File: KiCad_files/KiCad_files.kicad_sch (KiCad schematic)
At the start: 87 parts, among them J1 Conn_01x02_Socket, J10 MB1, J10 MB2, J13 MB1, J14 MB1, J16 MB2, J3 Conn_01x03_Socket, J6 Conn_01x01_Socket, J7 Conn_01x01_Socket, J8 Conn_01x01_Socket, J8 MB1, J8 MB2, J9 Conn_01x01_Socket, J9 MB1, J9 MB2, SW1 SW_Omron_B3FS, U2 LM22670QMR-5.0, U3 MC33275ST-3.3T3G, U4 ADM3488ExR, U6 LT1789

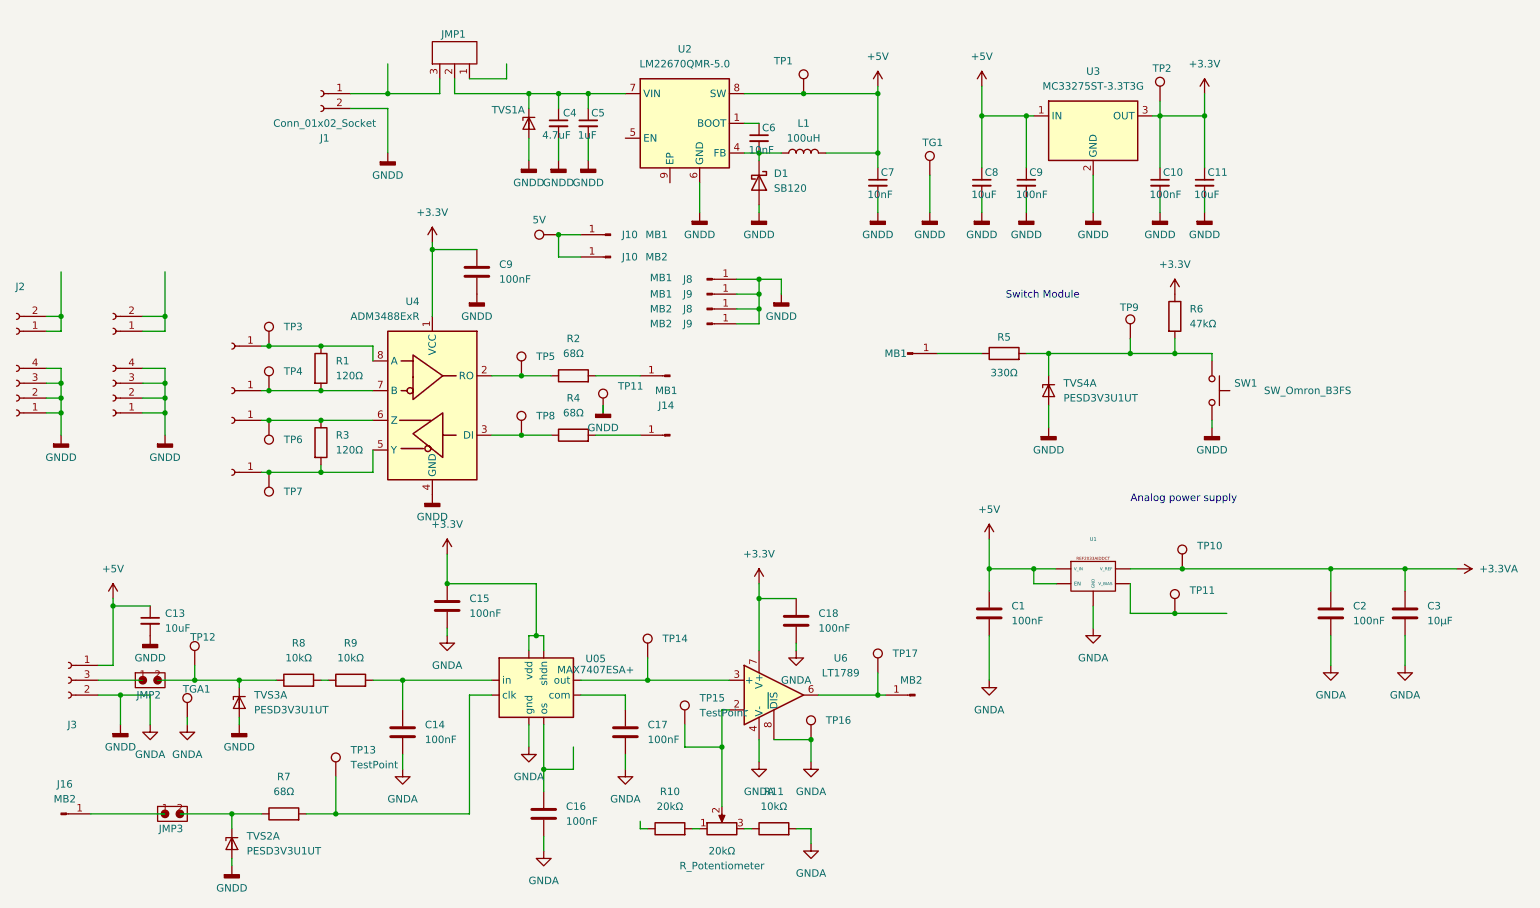
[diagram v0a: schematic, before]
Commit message: i inserted some footprints
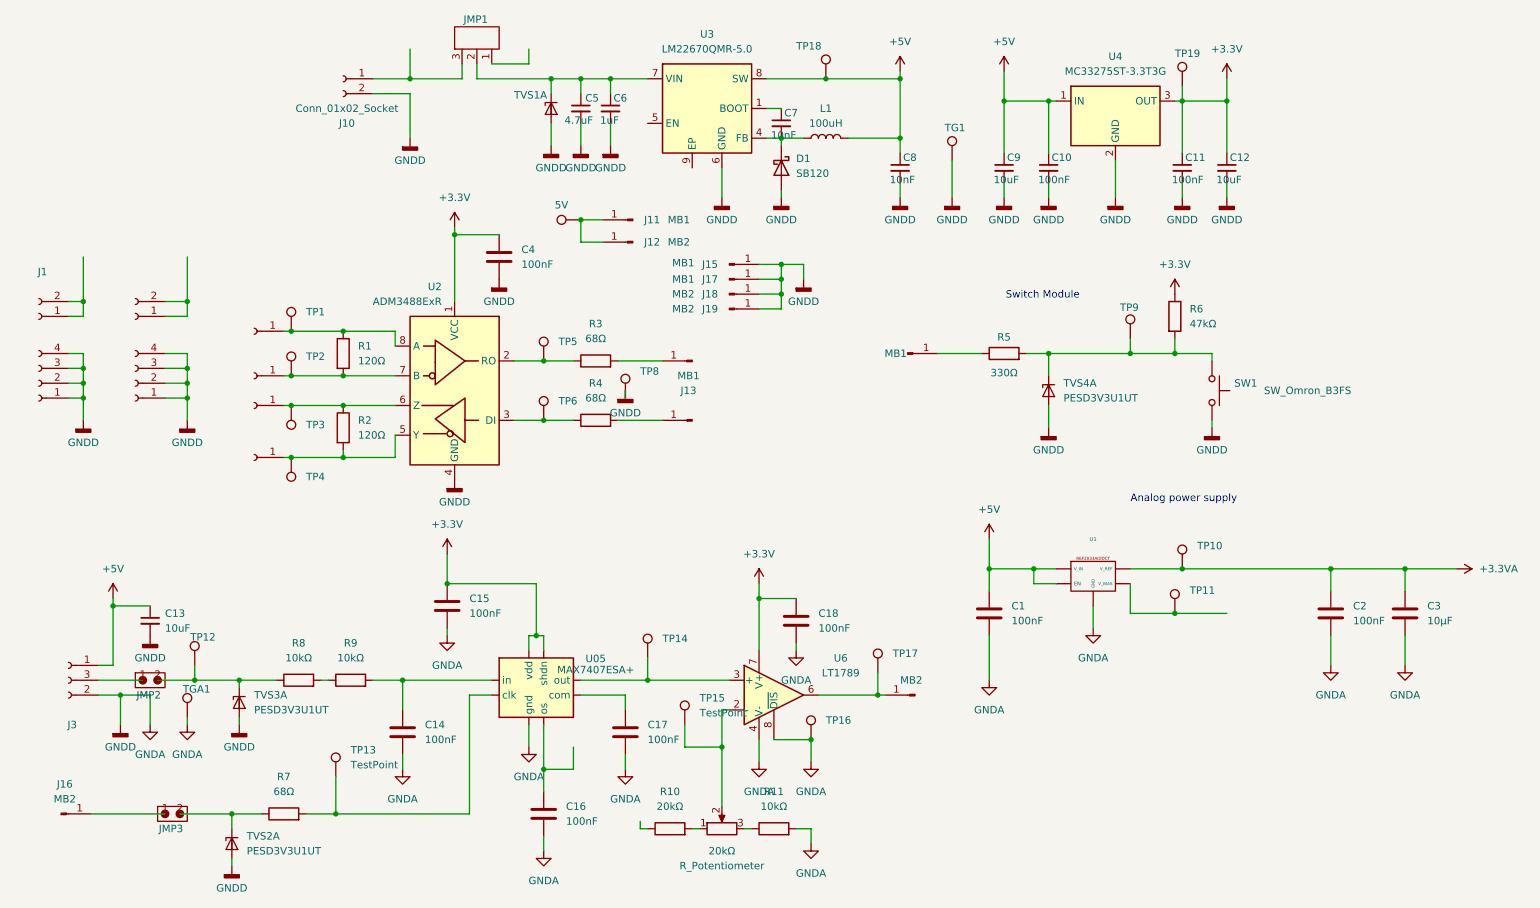
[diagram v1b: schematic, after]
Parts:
- removed C4: 4.7uF, symbol Device:C_Small
- removed C9: 100nF, symbol Device:C
- removed J10, J8, J9: MB1, symbol Connector:Conn_01x01_Pin
- removed J10, J8, J9: MB2, symbol Connector:Conn_01x01_Pin
- removed J2: ~, symbol Connector:Conn_01x02_Socket
- removed J3: ~, symbol Connector:Conn_01x04_Socket
- removed TP11: TestPoint, symbol Connector:TestPoint
- removed U2: LM22670QMR-5.0, Package_SO:SOIC-8-1EP_3.9x4.9mm_P1.27mm_EP2.29x3mm, symbol Regulator_Switching:LM22676MR-5
- removed U3: MC33275ST-3.3T3G, Package_TO_SOT_SMD:SOT-223, symbol Regulator_Linear:LT1963AxST-3.3
- removed U4: ADM3488ExR, Package_SO:SOIC-8_3.9x4.9mm_P1.27mm, symbol Interface_UART:ADM3488ExR
- added C12: 10uF, Capacitor_SMD:C_1210_3225Metric_Pad1.33x2.70mm_HandSolder, symbol Device:C_Small
- added C4: 100nF, symbol Device:C
- added J10: Conn_01x02_Socket, symbol Connector:Conn_01x02_Socket
- added J11, J15, J17: MB1, symbol Connector:Conn_01x01_Pin
- added J12, J18, J19: MB2, symbol Connector:Conn_01x01_Pin
- added J2: ~, symbol Connector:Conn_01x04_Socket
- added TP19: TestPoint, symbol Connector:TestPoint
- added U2: ADM3488ExR, Package_SO:SOIC-8_3.9x4.9mm_P1.27mm, symbol Interface_UART:ADM3488ExR
- added U3: LM22670QMR-5.0, Package_SO:SOIC-8-1EP_3.9x4.9mm_P1.27mm_EP2.29x3mm, symbol Regulator_Switching:LM22676MR-5
- added U4: MC33275ST-3.3T3G, Package_TO_SOT_SMD:SOT-223, symbol Regulator_Linear:LT1963AxST-3.3
- C10, C7: footprint (none) -> Capacitor_SMD:C_1206_3216Metric_Pad1.33x1.80mm_HandSolder
- C11: value 10uF -> 100nF; footprint (none) -> Capacitor_SMD:C_1206_3216Metric_Pad1.33x1.80mm_HandSolder
- C5: value 1uF -> 4.7uF; footprint (none) -> Capacitor_SMD:C_1206_3216Metric_Pad1.33x1.80mm_HandSolder
- C6: value 10nF -> 1uF; footprint (none) -> Capacitor_SMD:C_1206_3216Metric_Pad1.33x1.80mm_HandSolder
- C8: value 10uF -> 10nF; footprint (none) -> Capacitor_SMD:C_1206_3216Metric_Pad1.33x1.80mm_HandSolder
- C9: value 100nF -> 10uF; footprint (none) -> Capacitor_SMD:C_1210_3225Metric_Pad1.33x2.70mm_HandSolder
- J1: value Conn_01x02_Socket -> ~
- JMP1: footprint (none) -> Jumper:Pin_Header_2x1_P2.54mm_Vertical
- R1, R4: footprint (none) -> Resistor_SMD:R_1206_3216Metric_Pad1.30x1.75mm_HandSolder
- R2: value 68Ω -> 120Ω; footprint (none) -> Resistor_SMD:R_1206_3216Metric_Pad1.30x1.75mm_HandSolder
- R3: value 120Ω -> 68Ω; footprint (none) -> Resistor_SMD:R_1206_3216Metric_Pad1.30x1.75mm_HandSolder
- TP18: value 5V -> TestPoint
- TP7: value TestPoint -> 5V
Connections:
- net +3.3V: now also C12.1, C4.1, TP19.1, U2.1 (VCC), U4.3 (OUT); no longer C10.1, TP2.1
- net +5V: now also C10.1, TP18.1, U3.8 (SW), U4.1 (IN); no longer C7.1, TP1.1
- net GNDA: now also C6.2, TP8.1, C12.2, C4.2, J10.2 (Pin_2), J15.1 (Pin_1), J17.1 (Pin_1), J18.1 (Pin_1), J19.1 (Pin_1), J2.1 (Pin_1), J2.2 (Pin_2), J2.3 (Pin_3), J2.4 (Pin_4), U2.4 (GND), U3.6 (GND), U4.2 (GND); no longer C7.2, J1.2 (Pin_2)
- net at R4.1: now also TP6.1, U2.3 (DI); no longer TP8.1
- net at J13.1 (Pin_1): now also R3.2; no longer R4.2
- net at J6.1 (Pin_1), R1.1: now also TP1.1, U2.8 (A); no longer TP3.1
- net at J7.1 (Pin_1), R1.2: now also TP2.1, U2.7 (B); no longer TP4.1
- net at R2.1: now also J8.1 (Pin_1), TP3.1, U2.6 (Z); no longer TP5.1
- net at R2.2: now also J9.1 (Pin_1), TP4.1, U2.5 (Y); no longer J14.1 (Pin_1)
- net at C5.1, JMP1.2, TVS1.1 (K1): now also C6.1, U3.7 (VIN)
- net at J1.1 (Pin_1): now also J1.2 (Pin_2); no longer JMP1.3
- net at D1.1 (K), L1.1: now also C7.2, U3.4 (FB); no longer C6.2
- new net: R3.1, TP5.1, U2.2 (RO)
- new net: C7.1, U3.1 (BOOT)
- new net: J11.1 (Pin_1), J12.1 (Pin_1), TP7.1
- new net: J10.1 (Pin_1), JMP1.3
- new net: J14.1 (Pin_1), R4.2
